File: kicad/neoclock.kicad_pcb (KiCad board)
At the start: 2 copper layers, 51.3 x 23.9 mm, 31 parts, among them CON1 2.1mm 5V, IC1 ATMEGA328P-MM, K1 NEOPIXEL, P1 ICSP, P2 FTDI, SW1 H, SW2 M, U1 DS1307, X1 16Mhz, X2 32.768kHz

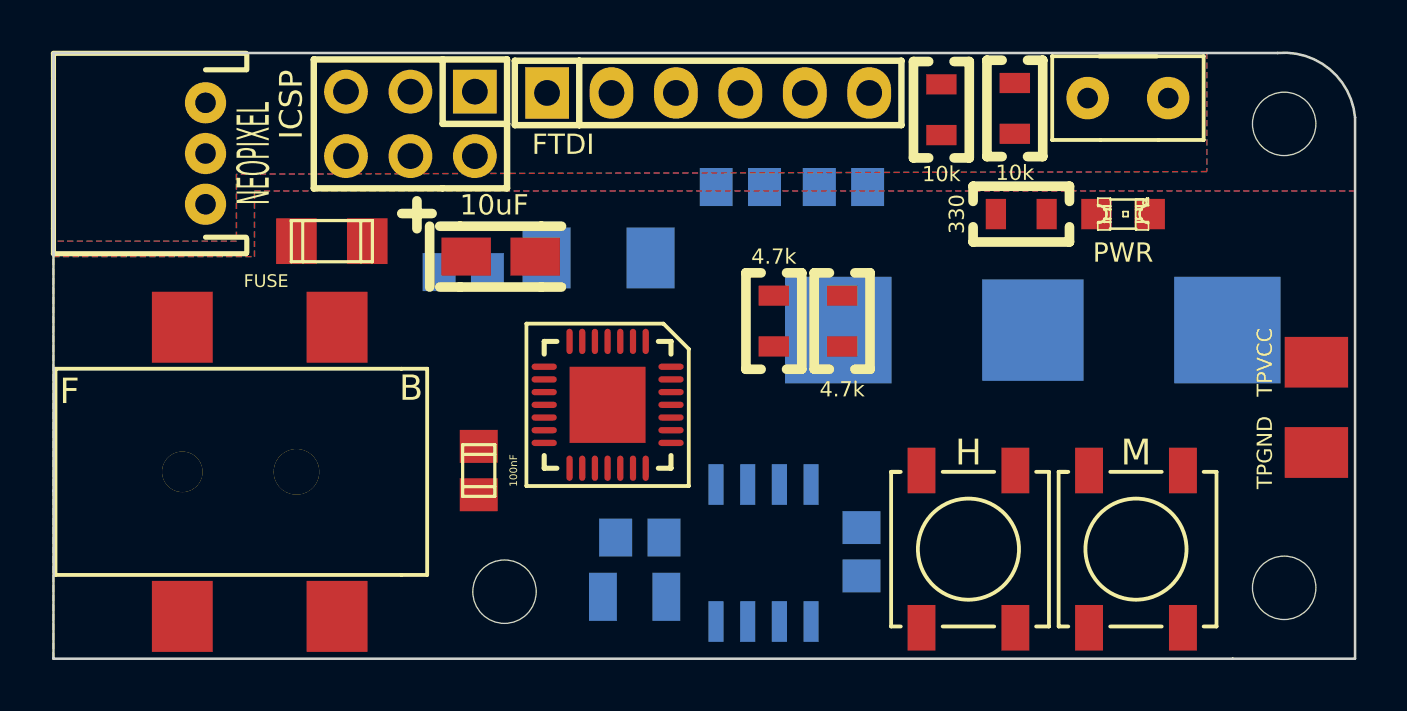
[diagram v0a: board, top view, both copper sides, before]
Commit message: all routed
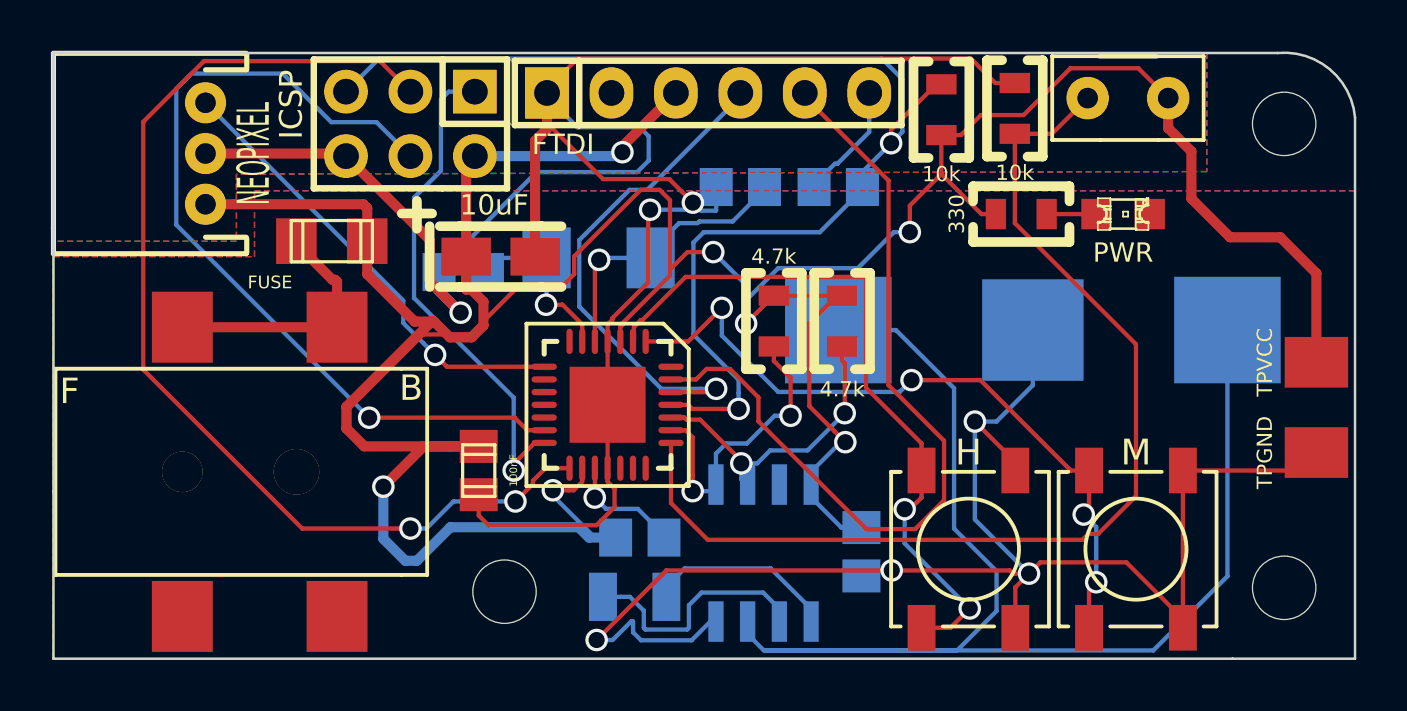
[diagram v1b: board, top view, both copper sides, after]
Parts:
- moved C3 0.20 mm to (55.1, 40.3)
- turned F1 to 180 degrees
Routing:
- net VCC: track 0.00 -> 157.0 mm, vias 0 -> 7
- net GND: track 0.00 -> 150.3 mm, vias 0 -> 7
- net Net-(BT1-Pad1): track 0.00 -> 55.4 mm
- net Net-(C3-Pad1): track 0.00 -> 48.6 mm, vias 0 -> 2
- net Net-(IC1-Pad15): track 0.00 -> 42.2 mm, vias 0 -> 2
- net Net-(IC1-Pad22): track 0.00 -> 41.7 mm
- net Net-(IC1-Pad13): track 0.00 -> 34.0 mm, vias 0 -> 1
- net Net-(IC1-Pad27): track 0.00 -> 32.9 mm
- net Net-(IC1-Pad1): track 0.00 -> 28.3 mm, vias 0 -> 4
- net Net-(IC1-Pad2): track 0.00 -> 28.2 mm, vias 0 -> 2
- net Net-(IC1-Pad26): track 0.00 -> 20.0 mm, vias 0 -> 1
- net Net-(IC1-Pad14): track 0.00 -> 20.0 mm, vias 0 -> 1
- net Net-(IC1-Pad8): track 0.00 -> 18.2 mm, vias 0 -> 1
- net I2CSCL: track 0.00 -> 12.1 mm, vias 0 -> 2
- net I2CSDA: track 0.00 -> 11.9 mm, vias 0 -> 2
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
